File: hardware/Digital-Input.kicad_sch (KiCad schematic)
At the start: 0 parts

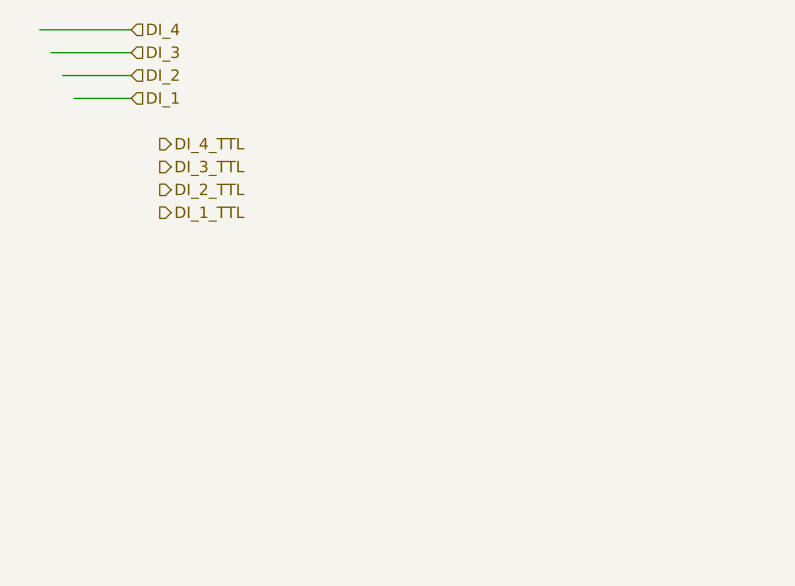
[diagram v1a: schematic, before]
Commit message: Layout updates
Signed-off-by: Connor Rigby <connorr@hey.com>
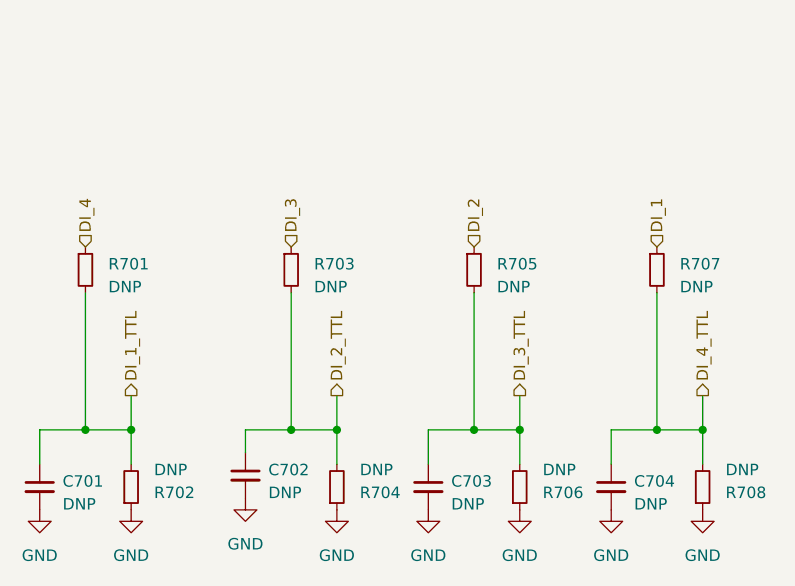
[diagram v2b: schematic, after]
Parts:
- added C701, C702, C703, C704: C_0603_DNP, Capacitor_SMD:C_0603_1608Metric, symbol LCSC_Capacitor:C_0603_DNP
- added R701, R702, R703, R704, R705, R706, R707, R708: DNP, Resistor_SMD:R_0603_1608Metric, symbol LCSC_Resistor:R_0603_DNP
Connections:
- net DI_1: now also R707.1
- net DI_1_TTL: now also C701.1, R701.2, R702.2
- net DI_2: now also R705.1
- net DI_2_TTL: now also C702.1, R703.2, R704.2
- net DI_3: now also R703.1
- net DI_3_TTL: now also C703.1, R705.2, R706.2
- net DI_4: now also R701.1
- net DI_4_TTL: now also C704.1, R707.2, R708.2
- new net GND: C701.2, C702.2, C703.2, C704.2, R702.1, R704.1, R706.1, R708.1
